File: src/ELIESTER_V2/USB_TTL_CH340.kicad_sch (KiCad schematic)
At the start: 26 parts, among them J5 USB_B_Micro, Q1 MMBT3904, Q2 MMBT3904, U4 CH340T(SSOP20W), Y1 12MHz

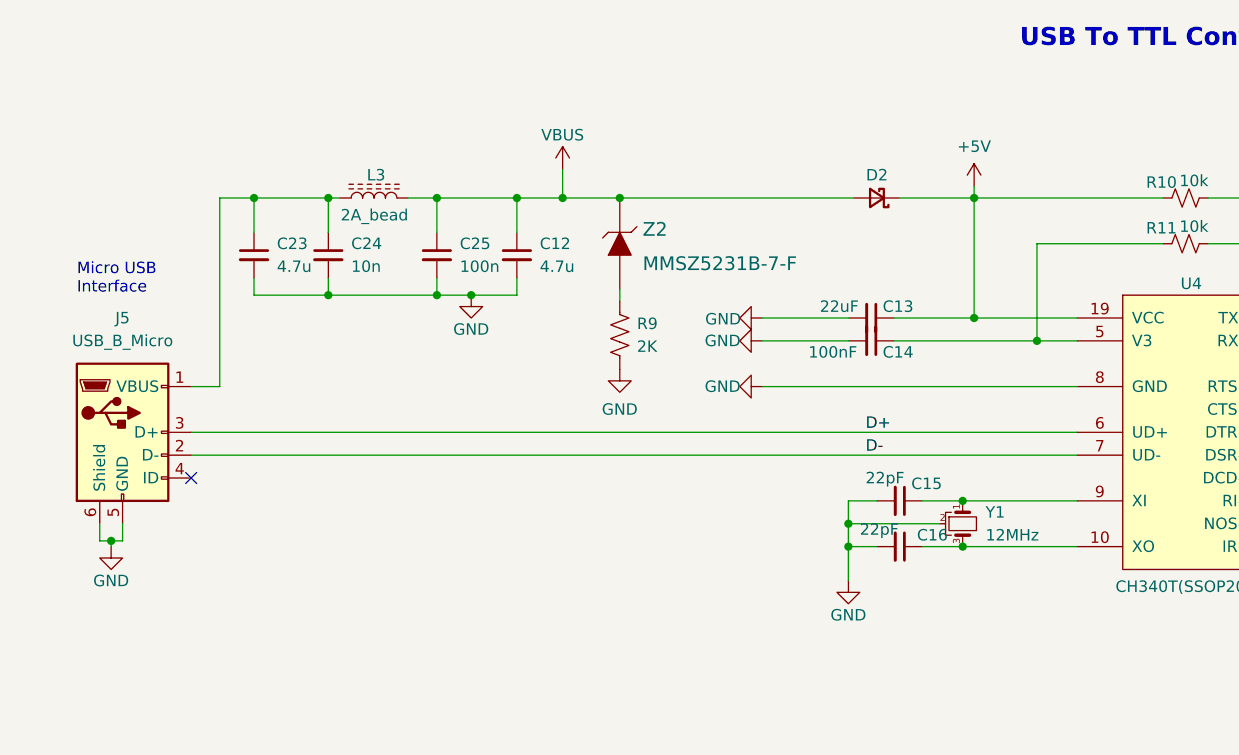
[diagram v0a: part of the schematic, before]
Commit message: schematic update and gerber updates with corrections
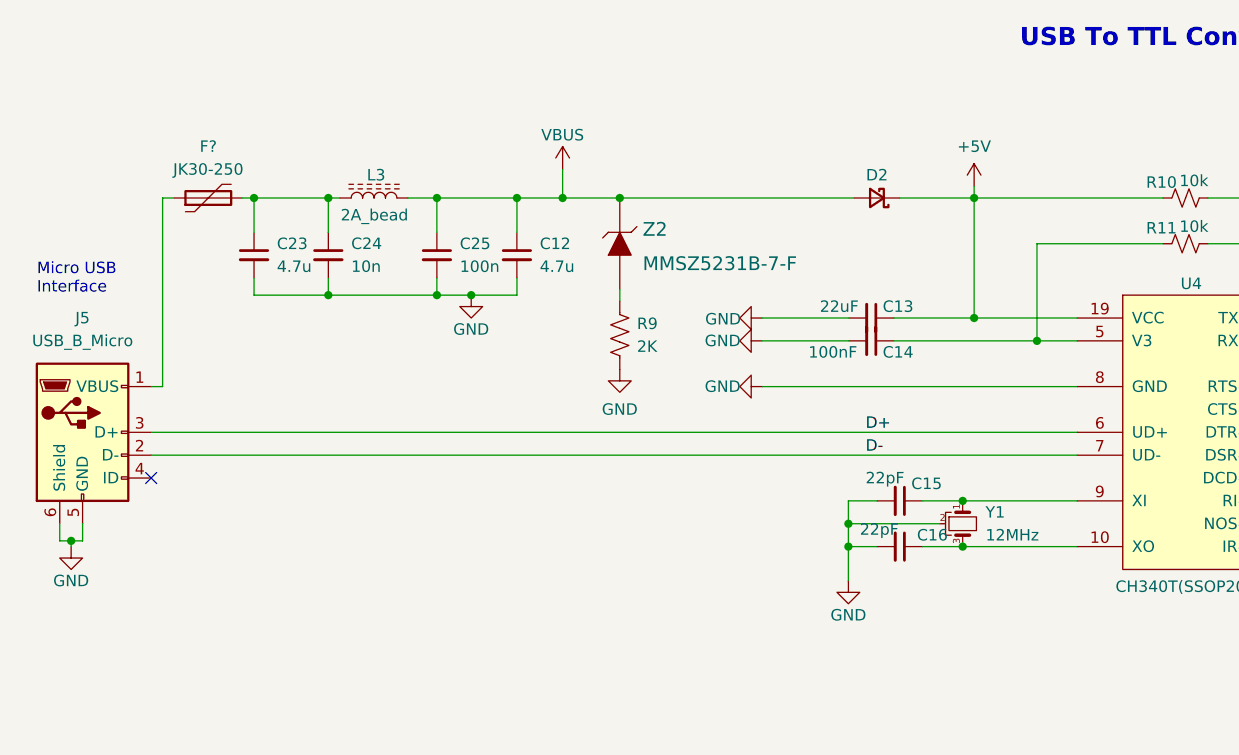
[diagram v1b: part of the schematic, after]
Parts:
- added F?: JK30-250, Fuse:Fuse_1210_3225Metric_Pad1.42x2.65mm_HandSolder, symbol Device:Polyfuse
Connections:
- net at C23.1, C24.1, L3.2: now also F?.2; no longer J5.1 (VBUS)
- new net: F?.1, J5.1 (VBUS)
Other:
- moved on the sheet: J5
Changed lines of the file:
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@@
     (comment 4 "ELIESTAR")
   )
-  (junction (at 22.225 109.855) (diameter 0) (color 0 0 0 0)
+  (junction (at 17.78 109.855) (diameter 0) (color 0 0 0 0)
   )
   (junction (at 67.31 71.755) (diameter 0) (color 0 0 0 0)
@@
   )
   (no_connect (at 154.94 100.33))
-  (no_connect (at 31.115 102.87))
+  (no_connect (at 26.67 102.87))
   (no_connect (at 154.94 95.25))
   (no_connect (at 154.94 102.87))
@@
     (stroke (width 0) (type default))
   )
+  (wire (pts (xy 36.83 71.755) (xy 38.1 71.755))
+    (stroke (width 0) (type default))
+  )
   (wire (pts (xy 199.39 102.87) (xy 199.39 104.775))
     (stroke (width 0) (type default))
   )
-  (wire (pts (xy 22.225 109.855) (xy 22.225 110.49))
+  (wire (pts (xy 17.78 109.855) (xy 17.78 110.49))
     (stroke (width 0) (type default))
   )
@@
     (stroke (width 0) (type default))
   )
-  (wire (pts (xy 22.225 109.855) (xy 23.495 109.855))
+  (wire (pts (xy 17.78 109.855) (xy 19.05 109.855))
     (stroke (width 0) (type default))
   )
@@
     (stroke (width 0) (type default))
   )
-  (wire (pts (xy 34.29 71.755) (xy 38.1 71.755))
+  (wire (pts (xy 27.94 71.755) (xy 29.21 71.755))
     (stroke (width 0) (type default))
   )
@@
     (stroke (width 0) (type default))
   )
-  (wire (pts (xy 31.115 100.33) (xy 129.54 100.33))
+  (wire (pts (xy 26.67 100.33) (xy 129.54 100.33))
     (stroke (width 0) (type default))
   )
@@
     (stroke (width 0) (type default))
   )
-  (wire (pts (xy 34.29 71.755) (xy 34.29 92.71))
+  (wire (pts (xy 27.94 71.755) (xy 27.94 92.71))
     (stroke (width 0) (type default))
   )
@@
     (stroke (width 0) (type default))
   )
-  (wire (pts (xy 34.29 92.71) (xy 31.115 92.71))
+  (wire (pts (xy 27.94 92.71) (xy 26.67 92.71))
     (stroke (width 0) (type default))
   )
@@
     (stroke (width 0) (type default))
   )
-  (wire (pts (xy 31.115 97.79) (xy 129.54 97.79))
+  (wire (pts (xy 26.67 97.79) (xy 129.54 97.79))
     (stroke (width 0) (type default))
   )
@@
     (stroke (width 0) (type default))
   )
-  (wire (pts (xy 20.955 107.95) (xy 20.955 109.855))
+  (wire (pts (xy 16.51 107.95) (xy 16.51 109.855))
     (stroke (width 0) (type default))
   )
@@
     (stroke (width 0) (type default))
   )
-  (wire (pts (xy 20.955 109.855) (xy 22.225 109.855))
+  (wire (pts (xy 16.51 109.855) (xy 17.78 109.855))
     (stroke (width 0) (type default))
   )
@@
     (stroke (width 0) (type default))
   )
-  (wire (pts (xy 23.495 107.95) (xy 23.495 109.855))
+  (wire (pts (xy 19.05 107.95) (xy 19.05 109.855))
     (stroke (width 0) (type default))
   )
@@
     (effects (font (size 1.27 1.27)) (justify left bottom))
   )
-  (text "Micro USB\nInterface" (at 18.415 82.55 0)
+  (text "Micro USB\nInterface" (at 13.97 82.55 0)
     (effects (font (size 1.27 1.27)) (justify left bottom))
   )
@@
         (path "/efe55700-0211-4481-aa01-7a7eb74def17/d31c3b4c-fc14-4a71-8e61-c96847deaf5b"
           (reference "#PWR033") (unit 1)
+        )
+      )
+    )
+  )
+  (symbol (lib_id "Device:Polyfuse") (at 33.02 71.755 90) (unit 1)
+    (in_bom yes) (on_board yes) (dnp no) (fields_autoplaced)
+    (property "Reference" "F?" (at 33.02 66.04 90)
+      (effects (font (size 1.27 1.27)))
+    )
+    (property "Value" "JK30-250" (at 33.02 68.58 90)
+      (effects (font (size 1.27 1.27)))
+    )
+    (property "Footprint" "Fuse:Fuse_1210_3225Metric_Pad1.42x2.65mm_HandSolder" (at 38.1 70.485 0)
+      (effects (font (size 1.27 1.27)) (justify left) hide)
+    )
+    (property "Datasheet" "~" (at 33.02 71.755 0)
+      (effects (font (size 1.27 1.27)) hide)
+    )
+    (pin "1")
+    (pin "2")
+    (instances
+      (project "ELIESTER_V2"
+        (path "/efe55700-0211-4481-aa01-7a7eb74def17"
+          (reference "F?") (unit 1)
+        )
+        (path "/efe55700-0211-4481-aa01-7a7eb74def17/d31c3b4c-fc14-4a71-8e61-c96847deaf5b"
+          (reference "F2") (unit 1)
         )
       )
@@
     )
   )
-  (symbol (lib_id "power:GND") (at 22.225 110.49 0) (unit 1)
-    (in_bom yes) (on_board yes) (dnp no)
-    (property "Reference" "#PWR025" (at 22.225 116.84 0)
-      (effects (font (size 1.27 1.27)) hide)
-    )
-    (property "Value" "GND" (at 22.225 114.3 0)
-      (effects (font (size 1.27 1.27)))
-    )
-    (property "Footprint" "" (at 22.225 110.49 0)
-      (effects (font (size 1.27 1.27)) hide)
-    )
-    (property "Datasheet" "" (at 22.225 110.49 0)
+  (symbol (lib_id "power:GND") (at 17.78 110.49 0) (unit 1)
+    (in_bom yes) (on_board yes) (dnp no)
+    (property "Reference" "#PWR025" (at 17.78 116.84 0)
+      (effects (font (size 1.27 1.27)) hide)
+    )
+    (property "Value" "GND" (at 17.78 114.3 0)
+      (effects (font (size 1.27 1.27)))
+    )
+    (property "Footprint" "" (at 17.78 110.49 0)
+      (effects (font (size 1.27 1.27)) hide)
+    )
+    (property "Datasheet" "" (at 17.78 110.49 0)
       (effects (font (size 1.27 1.27)) hide)
     )
@@
     )
   )
-  (symbol (lib_id "Connector:USB_B_Micro") (at 23.495 97.79 0) (unit 1)
+  (symbol (lib_id "Connector:USB_B_Micro") (at 19.05 97.79 0) (unit 1)
     (in_bom yes) (on_board yes) (dnp no) (fields_autoplaced)
-    (property "Reference" "J5" (at 23.495 85.09 0)
-      (effects (font (size 1.27 1.27)))
-    )
-    (property "Value" "USB_B_Micro" (at 23.495 87.63 0)
-      (effects (font (size 1.27 1.27)))
-    )
-    (property "Footprint" "Connector_USB:USB_Micro-B_Molex-105017-0001" (at 27.305 99.06 0)
-      (effects (font (size 1.27 1.27)) hide)
-    )
-    (property "Datasheet" "~" (at 27.305 99.06 0)
-      (effects (font (size 1.27 1.27)) hide)
-    )
+    (property "Reference" "J5" (at 19.05 85.09 0)
+      (effects (font (size 1.27 1.27)))
+    )
+    (property "Value" "USB_B_Micro" (at 19.05 87.63 0)
+      (effects (font (size 1.27 1.27)))
+    )
+    (property "Footprint" "Connector_USB:USB_Micro-B_Molex-105017-0001" (at 22.86 99.06 0)
+      (effects (font (size 1.27 1.27)) hide)
+    )
+    (property "Datasheet" "~" (at 22.86 99.06 0)
+      (effects (font (size 1.27 1.27)) hide)
+    )
